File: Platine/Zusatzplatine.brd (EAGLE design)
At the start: 55.6 x 49.5 mm, 31 parts, among them X2 22-23-2081, X3 22-23-2081, X4 22-23-2101

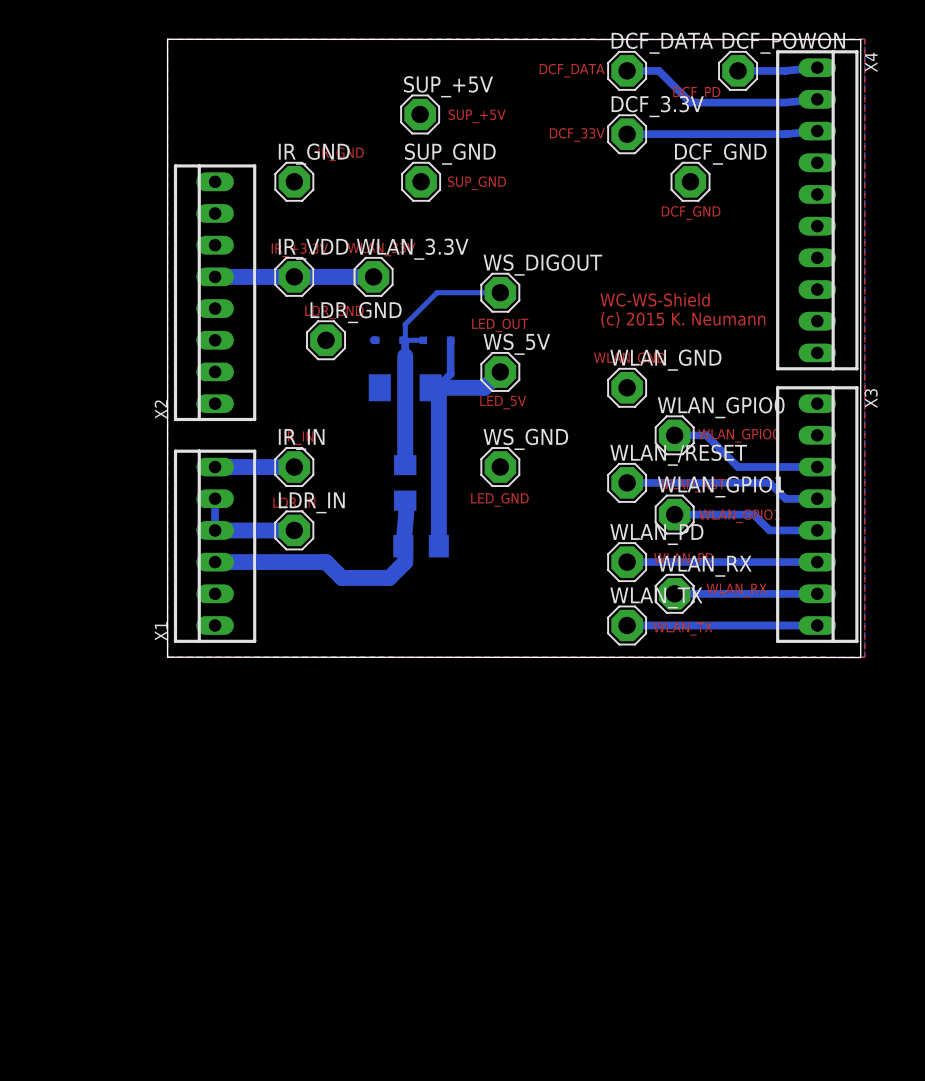
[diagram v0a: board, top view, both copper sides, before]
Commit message: Reworked Board Design
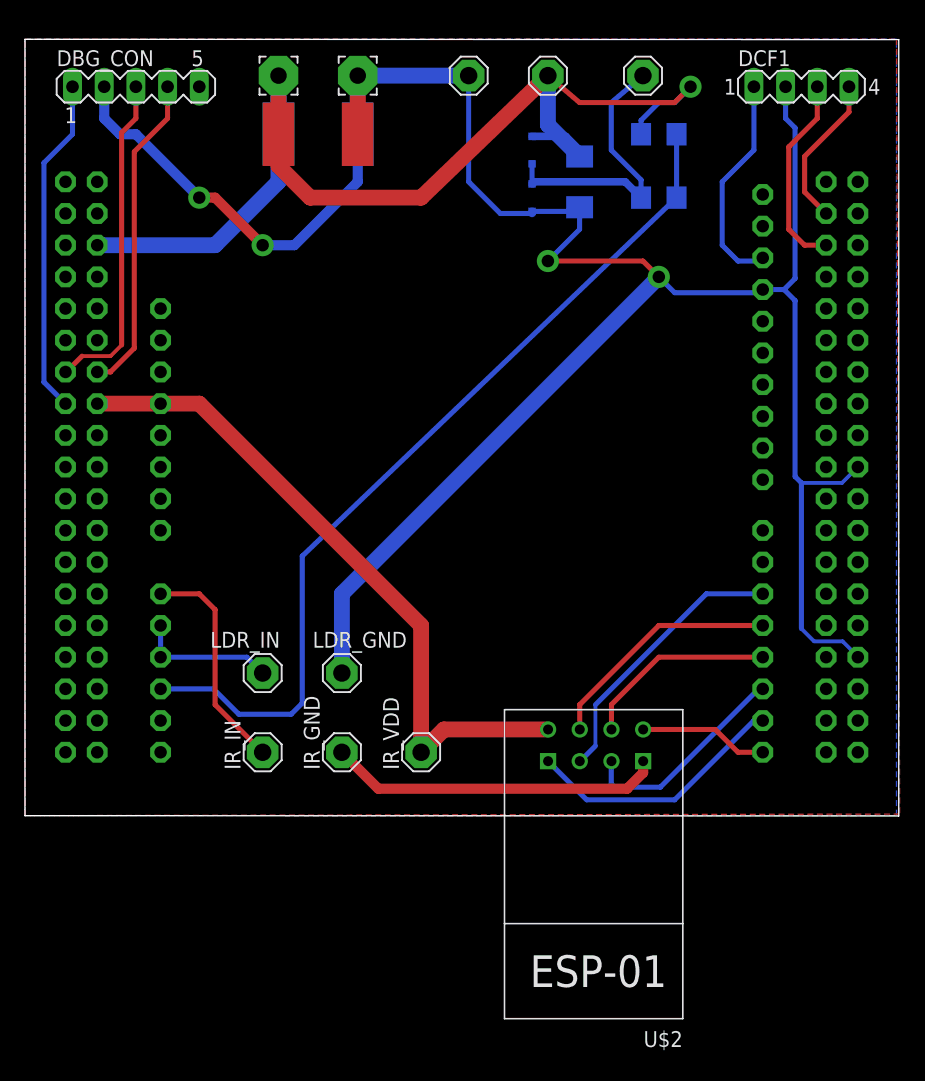
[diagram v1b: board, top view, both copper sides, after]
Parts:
- removed DCF_3.3V, DCF_DATA, DCF_GND, DCF_POWON, SUP_+5V, SUP_GND, WLAN_/RESET, WLAN_3.3V, WLAN_GND, WLAN_GPIO0, WLAN_GPIO1, WLAN_PD, WLAN_RX, WLAN_TX: SE14, solpad:SE14
- removed X1: (no value), con-molex:22-23-2061
- removed X2, X3: 22-23-2081, con-molex:22-23-2081
- removed X4: 22-23-2101, con-molex:22-23-2101
- added DBG_CON: (no value), con-lstb:MA05-1
- added DCF1: (no value), con-lstb:MA04-1
- added HOLE_EXT_+5V, HOLE_EXT_GND: WIREPAD3,17/1,3, wirepad:3,17/1,3
- added PAD_EXT_+5V, PAD_EXT_+5V1, PAD_EXT_GND, PAD_EXT_GND1: WIREPADSMD2,54-5,08, wirepad:SMD2,54-5,08
- added U$1: NUCLEO_F411RE, Stm32nucleo:NUCLEO_BRD64
- added U$2: ESP01, esp8266modules:ESP01
- moved IR_GND 45.9 mm to (25.4, 5.08), turned to 90 degrees
- moved IR_VDD 39.4 mm to (31.8, 5.08), turned to 90 degrees
- moved R2 38.1 mm to (50.8, 54.6)
- moved WS_GND 31.5 mm to (35.6, 59.3)
- moved R1 30.6 mm to (50.8, 49.5), turned to 0 degrees
- moved LDR_GND 26.7 mm to (25.4, 11.4), turned to 90 degrees
- moved WS_5V 24.1 mm to (41.9, 59.3)
- moved IR_IN 23.0 mm to (19.1, 5.08), turned to 90 degrees
- moved D4 21.6 mm to (44.5, 50.8), turned to 270 degrees
- moved WS_DIGOUT 20.8 mm to (49.5, 59.3)
- moved D1 17.0 mm to (40.6, 53.3), turned to 90 degrees
- moved D2 16.2 mm to (40.6, 49.5), turned to 90 degrees
- moved LDR_IN 11.7 mm to (19.1, 11.4), turned to 90 degrees
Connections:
- removed net +3.3V: IR_VDD.MP, WLAN_3.3V.MP, X2.5
- removed net N$10: DCF_POWON.MP, X4.1
- removed net N$11: DCF_DATA.MP, X4.2
- removed net N$3: LDR_IN.MP, X1.4, X1.5
- removed net N$4: WLAN_RX.MP, X3.7
- removed net N$5: WLAN_PD.MP, X3.6
- removed net N$6: WLAN_GPIO1.MP, X3.5
- removed net N$7: WLAN_/RESET.MP, X3.4
- removed net N$9: WLAN_GPIO0.MP, X3.3
- new net +3V3: IR_VDD.MP, U$1.3V, U$1.3V3, U$2.VCC
- new net DCF1_DATA: DCF1.3, U$1.PB9
- new net DCF1_PON: DCF1.4, U$1.PB8
- new net GND1: U$1.GND1
- new net GND2: U$1.GND2
- new net GND3: U$1.GND3
- new net GND4: U$1.GND4
- new net GND5: U$1.GND5
- new net GND6: U$1.GND6
- new net GND7: U$1.GND7
- new net IR_IN: IR_IN.MP, U$1.A0
- new net LDR_IN: LDR_IN.MP, U$1.A1, U$1.A2
- new net N$12: U$1.D5, U$2.GPIO0
- new net N$13: U$1.D4, U$2.RST
- new net N$14: U$1.D3, U$2.CH_PD
- new net N$15: U$1.D0, U$2.TX
- new net N$16: U$1.D1, U$2.RX
- new net N$17: U$1.D2, U$2.GPIO2
- new net NRST: DBG_CON.4, U$1.NRESET
- new net SWCLK: DBG_CON.1, U$1.PA14
- new net SWDIO: DBG_CON.3, U$1.PA13
- new net SWO: DBG_CON.5
- new net U5V: U$1.U5V
- new net VBAT: U$1.VBAT
- new net VDD: U$1.VDD
- new net VIN: U$1.VIN
- new net VIN2: U$1.VIN2
- net +5V: now also HOLE_EXT_+5V.1, PAD_EXT_+5V.1, PAD_EXT_+5V1.1, R2.1, U$1.E5V; no longer R2.2, SUP_+5V.MP, X2.4
- net AVDD: now also U$1.AVDD; no longer DCF_3.3V.MP, X4.3
- net GND: now also DBG_CON.2, DCF1.2, HOLE_EXT_GND.1, PAD_EXT_GND.1, PAD_EXT_GND1.1, U$1.AGND, U$1.GND, U$1.GND8, U$2.GND; no longer DCF_GND.MP, SUP_GND.MP, X2.2, X2.3
- net LED-OUT: now also R2.2, U$1.A3; no longer R2.1, X1.3
- net N$1: now also DCF1.1, U$1.AREF; no longer WLAN_TX.MP, X3.8
- net N$2: now also U$1.5V, U$1.5V2; no longer IR_IN.MP, X1.6
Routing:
- net GND: track 0.17 -> 219.9 mm, vias 0 -> 4
- net +5V: track 23.1 -> 90.2 mm, vias 0 -> 1
- net +3V3: track 0.00 -> 54.4 mm
- net LED-OUT: track 21.4 -> 71.0 mm
- net SWCLK: track 0.00 -> 27.1 mm
- net SWDIO: track 0.00 -> 26.6 mm
- net NRST: track 0.00 -> 25.8 mm
- net N$12: track 0.00 -> 22.2 mm
- net N$16: track 0.00 -> 21.1 mm
- net N$13: track 0.00 -> 19.3 mm
- net IR_IN: track 0.00 -> 17.9 mm
- net N$17: track 0.00 -> 17.3 mm
- net N$11: track 16.3 -> 0.00 mm
- net DCF1_DATA: track 0.00 -> 15.9 mm
- net N$7: track 15.8 -> 0.00 mm
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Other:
- board size 55.6 x 49.5 mm -> 70 x 62.2 mm
- board text added: "5V IN"
- board text added: "GND IN"
- board text added: "LED 5V"
- board text added: "LED GND"
- board text added: "LED SIG"
- board text added: "SUPPLY"
- board text added: "WC-WS-Shield for Nucleo (c) 2015 K. Neumann, J. Berg"
- board text removed: "DCF_33V"
- board text removed: "DCF_DATA"
- board text removed: "DCF_GND"
- board text removed: "DCF_PD"
- board text removed: "IR_+3.3V"
- board text removed: "IR_GND"
- board text removed: "IR_IN"
- board text removed: "LDR_GND"
- board text removed: "LDR_IN"
- board text removed: "LED_5V"
- board text removed: "LED_GND"
- board text removed: "LED_OUT"
- board text removed: "SUP_+5V"
- board text removed: "SUP_GND"
- board text removed: "WC-WS-Shield (c) 2015 K. Neumann"
- board text removed: "WLAN_33V"
- board text removed: "WLAN_GND"
- board text removed: "WLAN_GPIO0"
- board text removed: "WLAN_GPIO1"
- board text removed: "WLAN_PD"
- board text removed: "WLAN_RST"
- board text removed: "WLAN_RX"
- board text removed: "WLAN_TX"
